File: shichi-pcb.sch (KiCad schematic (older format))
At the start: 29 parts, among them J1 USB_C_Receptacle_HRO_TYPE-C-3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, J2 Conn_01x06_Male, J3 Conn_01x04_Male, SW1 SW_Push, SW2 SW_Push, U1 MCP1700-3302E_SOT23, U2 PRTR5V0U2X, U3 STM32F072CBTx

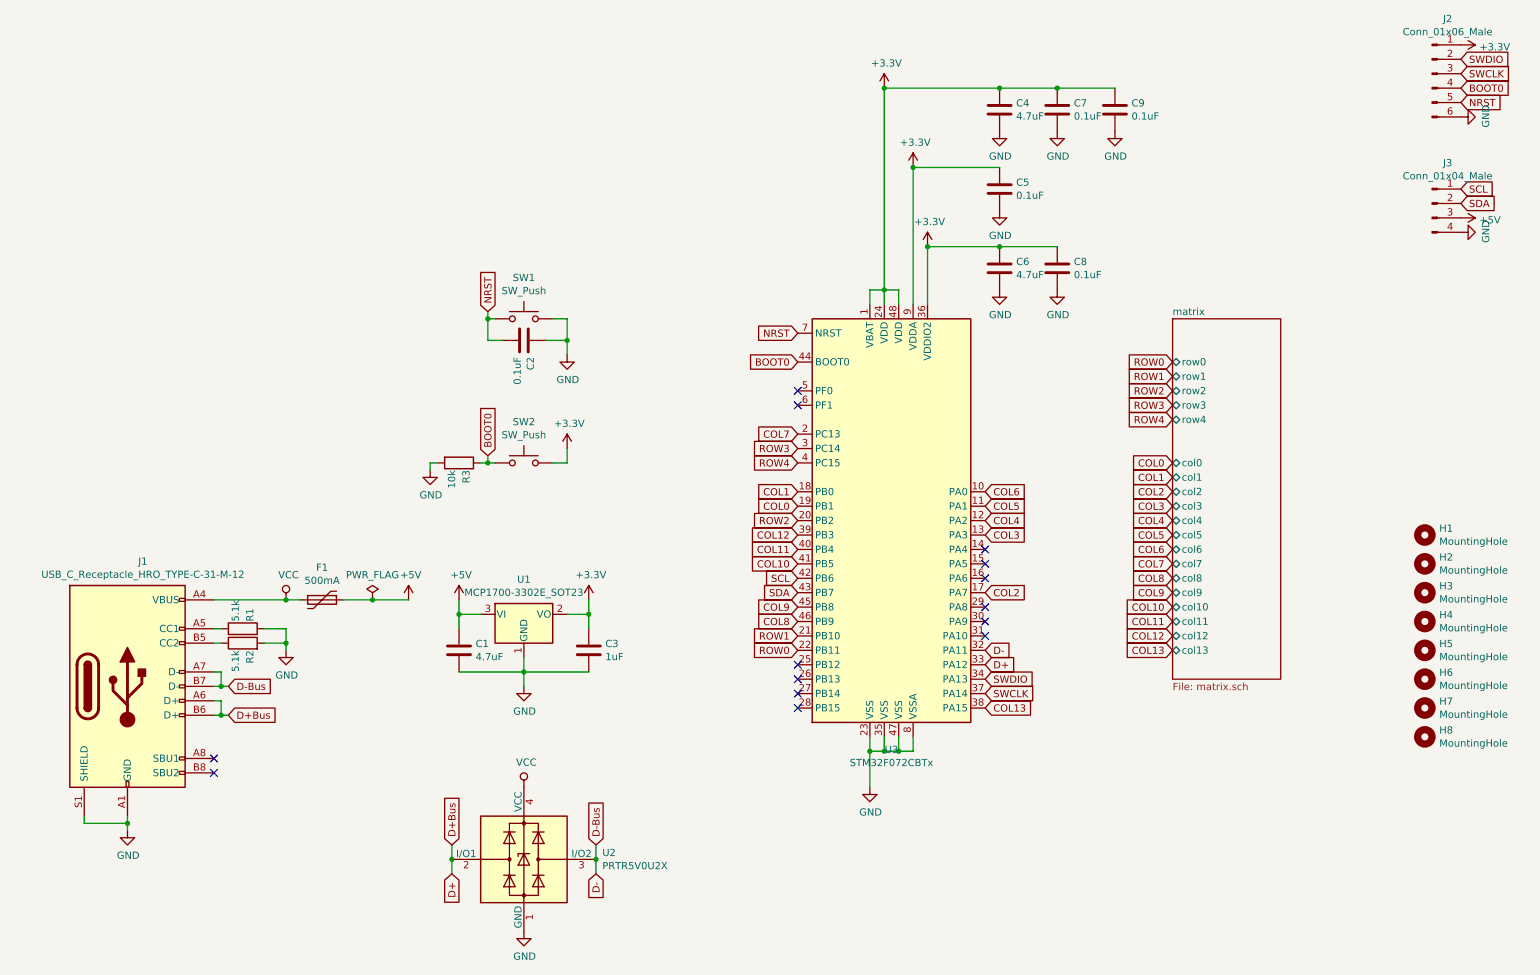
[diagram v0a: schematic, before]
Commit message: Optimize matrix pinout
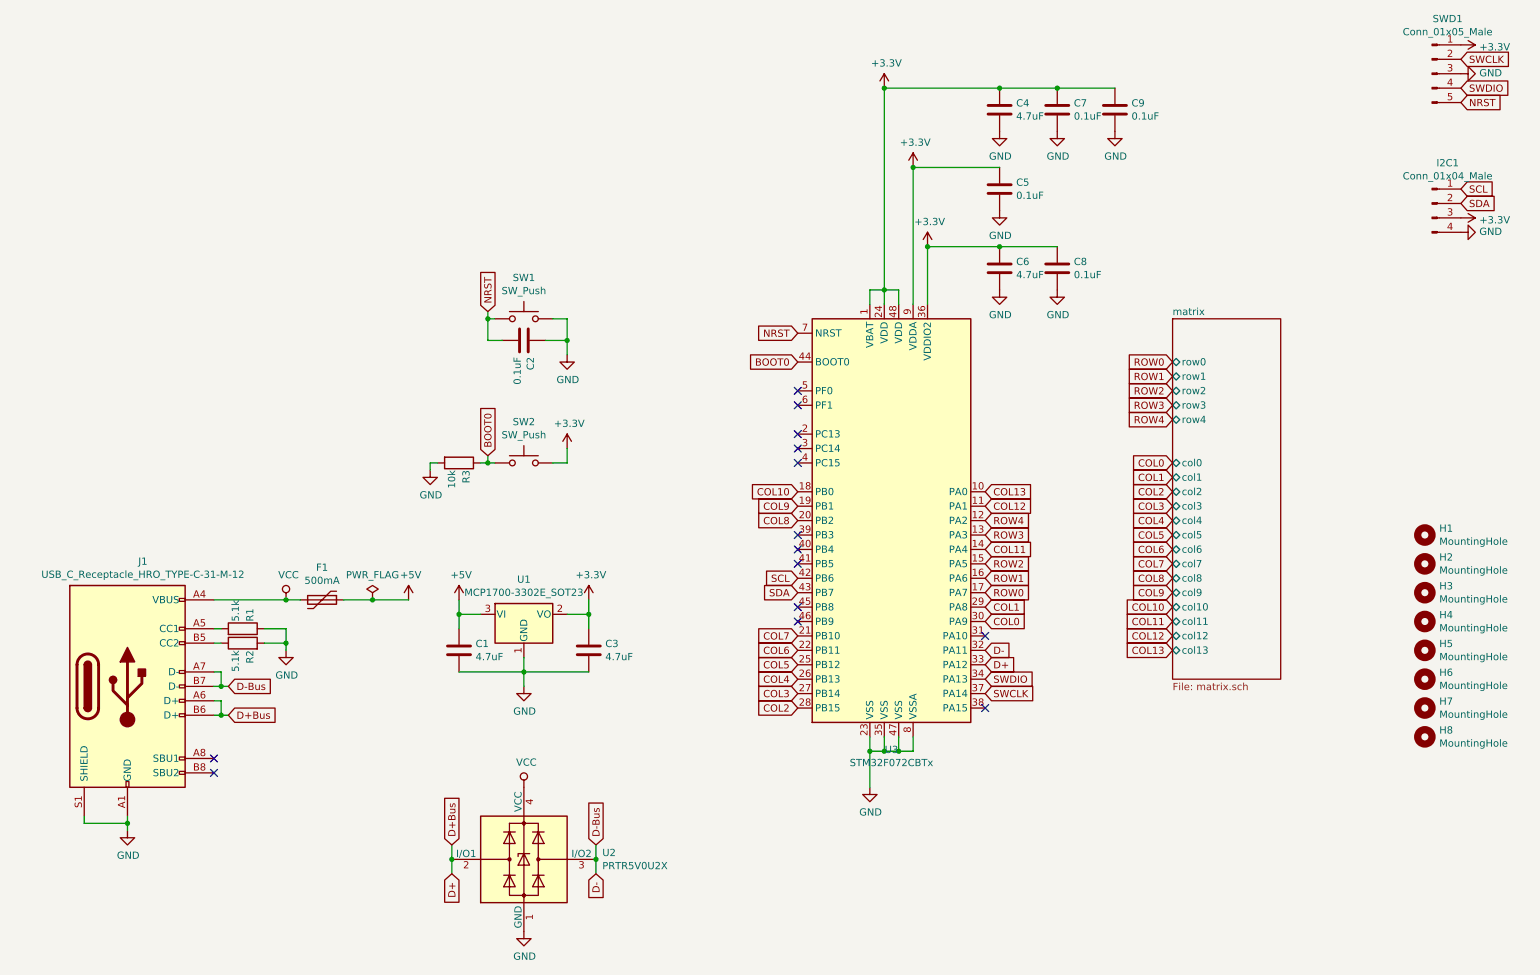
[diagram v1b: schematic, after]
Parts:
- removed J2: Conn_01x06_Male, Connector_PinSocket_2.54mm:PinSocket_1x06_P2.54mm_Vertical, symbol Connector:Conn_01x06_Male
- added SWD1: Conn_01x05_Male, Miscellaneous_Keyboard_Parts:SWD_Header_1x05_P2.54mm_Vertical, symbol Connector:Conn_01x05_Male
- C3: value 1uF -> 4.7uF
- I2C1: renamed from J3; footprint Connector_PinSocket_2.54mm:PinSocket_1x04_P2.54mm_Vertical -> Miscellaneous_Keyboard_Parts:I2C_Header_1x04_P2.54mm_Vertical
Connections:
- net +3V3: now also I2C1.3 (Pin_3), SWD1.1 (Pin_1)
- net +5V: no longer I2C1.3 (Pin_3)
- net COL0: now also U3.30 (PA9); no longer U3.19 (PB1)
- net COL1: now also U3.29 (PA8); no longer U3.18 (PB0)
- net COL10: now also U3.18 (PB0); no longer U3.41 (PB5)
- net COL11: now also U3.14 (PA4); no longer U3.40 (PB4)
- net COL12: now also U3.11 (PA1); no longer U3.39 (PB3)
- net COL13: now also U3.10 (PA0); no longer U3.38 (PA15)
- net COL2: now also U3.28 (PB15); no longer U3.17 (PA7)
- net COL3: now also U3.27 (PB14); no longer U3.13 (PA3)
- net COL4: now also U3.26 (PB13); no longer U3.12 (PA2)
- net COL5: now also U3.25 (PB12); no longer U3.11 (PA1)
- net COL6: now also U3.22 (PB11); no longer U3.10 (PA0)
- net COL7: now also U3.21 (PB10); no longer U3.2 (PC13)
- net COL8: now also U3.20 (PB2); no longer U3.46 (PB9)
- net COL9: now also U3.19 (PB1); no longer U3.45 (PB8)
- net GND: now also SWD1.3 (Pin_3)
- net NRST: now also SWD1.5 (Pin_5)
- net ROW0: now also U3.17 (PA7); no longer U3.22 (PB11)
- net ROW1: now also U3.16 (PA6); no longer U3.21 (PB10)
- net ROW2: now also U3.15 (PA5); no longer U3.20 (PB2)
- net ROW3: now also U3.13 (PA3); no longer U3.3 (PC14)
- net ROW4: now also U3.12 (PA2); no longer U3.4 (PC15)
- net SWCLK: now also SWD1.2 (Pin_2)
- net SWDIO: now also SWD1.4 (Pin_4)
